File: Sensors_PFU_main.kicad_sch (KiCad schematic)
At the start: 1 part, among them U1 AD797

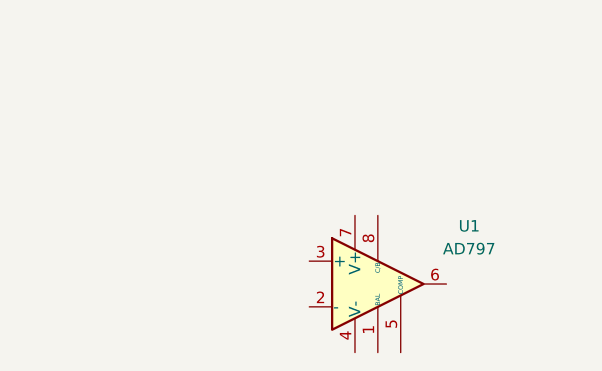
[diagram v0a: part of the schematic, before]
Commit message: Revert "modifico otro sch"
This reverts commit 6a0869d378a7460b569b04723fe4b47b4c436e1d.
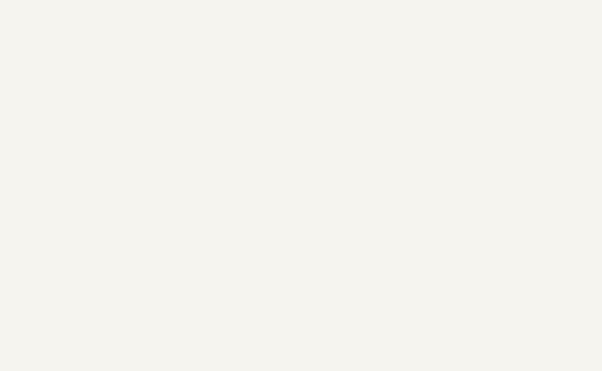
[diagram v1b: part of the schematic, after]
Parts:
- removed U1: AD797, symbol Amplifier_Operational:AD797
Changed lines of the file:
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@@
 		)
 	)
-	(symbol
-		(lib_id "Amplifier_Operational:AD797")
-		(at 138.43 125.73 0)
-		(unit 1)
-		(exclude_from_sim no)
-		(in_bom yes)
-		(on_board yes)
-		(dnp no)
-		(fields_autoplaced yes)
-		(property "Reference" "U1"
-			(at 148.59 119.3098 0)
-			(effects
-				(font
-					(size 1.27 1.27)
-				)
-			)
-		)
-		(property "Value" "AD797"
-			(at 148.59 121.8498 0)
-			(effects
-				(font
-					(size 1.27 1.27)
-				)
-			)
-		)
-		(property "Footprint" ""
-			(at 139.7 124.46 0)
-			(effects
-				(font
-					(size 1.27 1.27)
-				)
-				(hide yes)
-			)
-		)
-		(property "Datasheet" "https://www.analog.com/media/en/technical-documentation/data-sheets/AD797.pdf"
-			(at 139.7 121.92 0)
-			(effects
-				(font
-					(size 1.27 1.27)
-				)
-				(hide yes)
-			)
-		)
-		(property "Description" "Ultralow Distortion, Ultralow Noise Op Amp, DIP-8/SOIC-8"
-			(at 138.43 125.73 0)
-			(effects
-				(font
-					(size 1.27 1.27)
-				)
-				(hide yes)
-			)
-		)
-		(pin "6"
-		)
-		(pin "1"
-		)
-		(pin "7"
-		)
-		(pin "3"
-		)
-		(pin "4"
-		)
-		(pin "5"
-		)
-		(pin "2"
-		)
-		(pin "8"
-		)
-		(instances
-			(project ""
-				(path "/edac787c-3759-490a-b0c1-b3921b68d461"
-					(reference "U1")
-					(unit 1)
-				)
-			)
-		)
-	)
-	(sheet_instances
-		(path "/"
-			(page "1")
-		)
-	)
-	(embedded_fonts no)
 )

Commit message: modifico otro sch
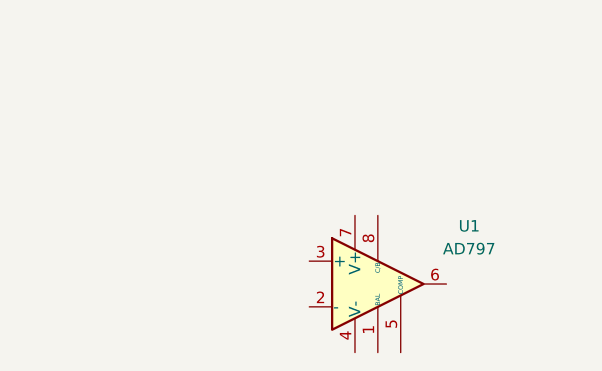
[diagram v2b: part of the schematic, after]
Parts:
- added U1: AD797, symbol Amplifier_Operational:AD797
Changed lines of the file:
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@@
 		)
 	)
+	(symbol
+		(lib_id "Amplifier_Operational:AD797")
+		(at 138.43 125.73 0)
+		(unit 1)
+		(exclude_from_sim no)
+		(in_bom yes)
+		(on_board yes)
+		(dnp no)
+		(fields_autoplaced yes)
+		(property "Reference" "U1"
+			(at 148.59 119.3098 0)
+			(effects
+				(font
+					(size 1.27 1.27)
+				)
+			)
+		)
+		(property "Value" "AD797"
+			(at 148.59 121.8498 0)
+			(effects
+				(font
+					(size 1.27 1.27)
+				)
+			)
+		)
+		(property "Footprint" ""
+			(at 139.7 124.46 0)
+			(effects
+				(font
+					(size 1.27 1.27)
+				)
+				(hide yes)
+			)
+		)
+		(property "Datasheet" "https://www.analog.com/media/en/technical-documentation/data-sheets/AD797.pdf"
+			(at 139.7 121.92 0)
+			(effects
+				(font
+					(size 1.27 1.27)
+				)
+				(hide yes)
+			)
+		)
+		(property "Description" "Ultralow Distortion, Ultralow Noise Op Amp, DIP-8/SOIC-8"
+			(at 138.43 125.73 0)
+			(effects
+				(font
+					(size 1.27 1.27)
+				)
+				(hide yes)
+			)
+		)
+		(pin "6"
+		)
+		(pin "1"
+		)
+		(pin "7"
+		)
+		(pin "3"
+		)
+		(pin "4"
+		)
+		(pin "5"
+		)
+		(pin "2"
+		)
+		(pin "8"
+		)
+		(instances
+			(project ""
+				(path "/edac787c-3759-490a-b0c1-b3921b68d461"
+					(reference "U1")
+					(unit 1)
+				)
+			)
+		)
+	)
+	(sheet_instances
+		(path "/"
+			(page "1")
+		)
+	)
+	(embedded_fonts no)
 )
